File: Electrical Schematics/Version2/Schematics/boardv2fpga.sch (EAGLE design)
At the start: 132 parts, among them Q1 ASFL1

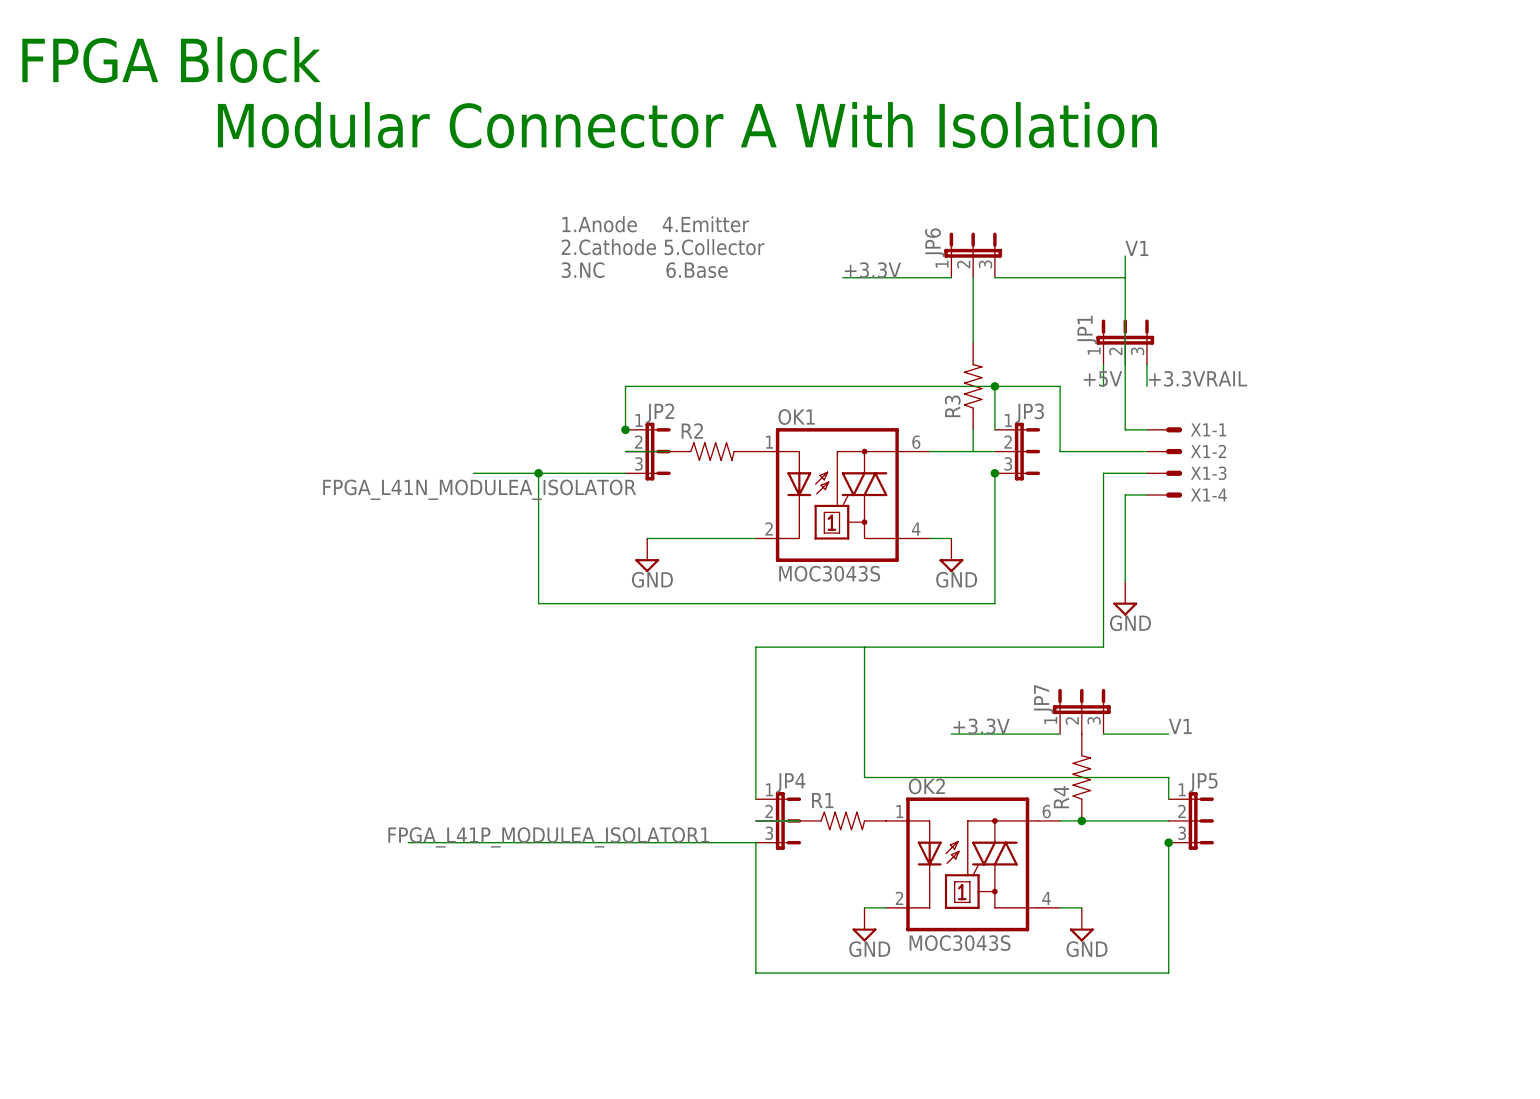
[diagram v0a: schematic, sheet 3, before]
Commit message: Fixed Grounds
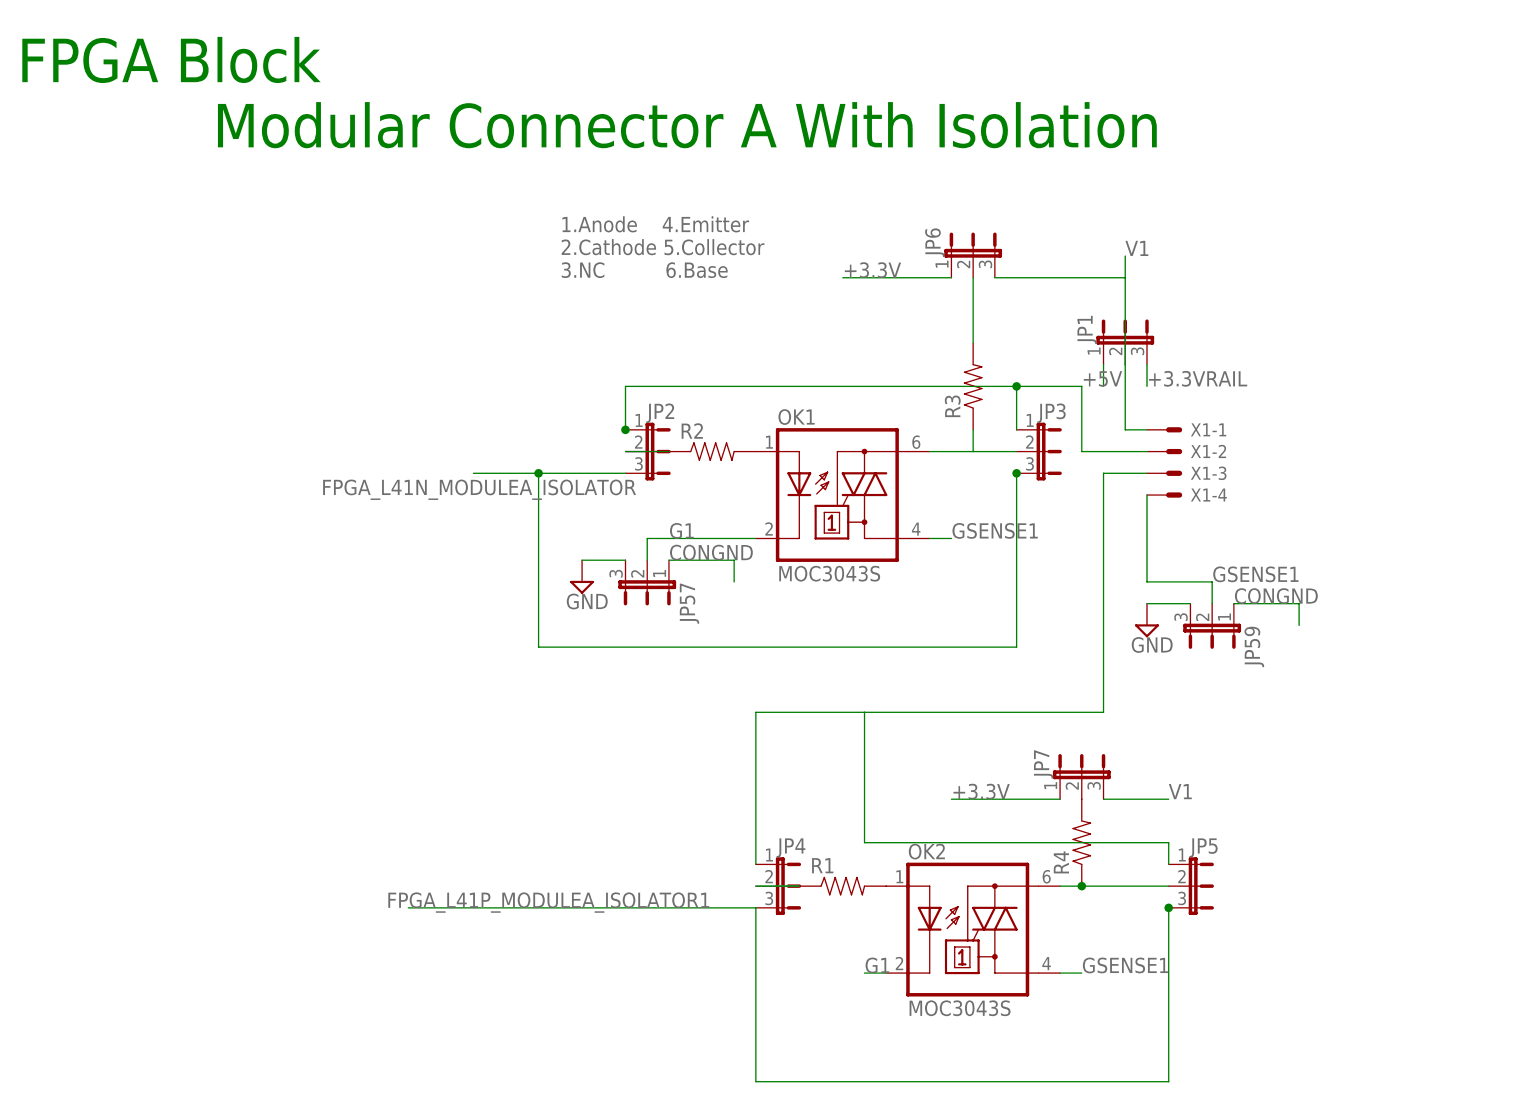
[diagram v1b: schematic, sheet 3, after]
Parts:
- added JP57, JP59, JP60, JP61, JP64, JP65, JP66, JP68, JP69, JP71, JP72, JP74, JP75, JP77, JP78, JP80: (no value), jumper:JP2E
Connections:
- new net CONGND: JP57.1, JP59.1, JP60.1, JP61.1, JP64.1, JP65.1, JP66.1, JP68.1, JP69.1, JP71.1, JP72.1, JP74.1, JP75.1, JP77.1, JP78.1, JP80.1
- new net G1: JP57.2, OK1.C, OK2.C
- new net G2: JP60.2, OK3.C, OK4.C
- new net G3: JP65.2, OK5.C, OK6.C
- new net G4: JP66.2, OK7.C, OK8.C
- new net G5: JP69.2, OK10.C, OK9.C
- new net G6: JP72.2, OK11.C, OK12.C
- new net G7: JP75.2, OK13.C, OK14.C
- new net G8: JP78.2, OK15.C, OK16.C
- new net GSENSE1: JP59.2, OK1.A1, OK2.A1, X1-4.S
- new net GSENSE2: JP61.2, OK3.A1, OK4.A1, X2-4.S
- new net GSENSE3: JP64.2, OK5.A1, OK6.A1, X3-4.S
- new net GSENSE4: JP68.2, OK7.A1, OK8.A1, X4-4.S
- new net GSENSE5: JP71.2, OK10.A1, OK9.A1, X5-4.S
- new net GSENSE6: JP74.2, OK11.A1, OK12.A1, X6-4.S
- new net GSENSE7: JP77.2, OK13.A1, OK14.A1, X7-4.S
- new net GSENSE8: JP80.2, OK15.A1, OK16.A1, X8-4.S
- net GND: now also JP57.3, JP59.3, JP60.3, JP61.3, JP64.3, JP65.3, JP66.3, JP68.3, JP69.3, JP71.3, JP72.3, JP74.3, JP75.3, JP77.3, JP78.3, JP80.3; no longer OK1.A1, OK1.C, OK10.A1, OK10.C, OK11.A1, OK11.C, OK12.A1, OK12.C, OK13.A1, OK13.C, OK14.A1, OK14.C, OK15.A1, OK15.C, OK16.A1, OK16.C, OK2.A1, OK2.C, OK3.A1, OK3.C, OK4.A1, OK4.C, OK5.A1, OK5.C, OK6.A1, OK6.C, OK7.A1, OK7.C, OK8.A1, OK8.C, OK9.A1, OK9.C, X1-4.S, X2-4.S, X3-4.S, X4-4.S, X5-4.S, X6-4.S, X7-4.S, X8-4.S
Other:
- moved on the sheet: JP11, JP12, JP14, JP18, JP19, JP21, JP25, JP26, JP28, JP3, JP32, JP33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

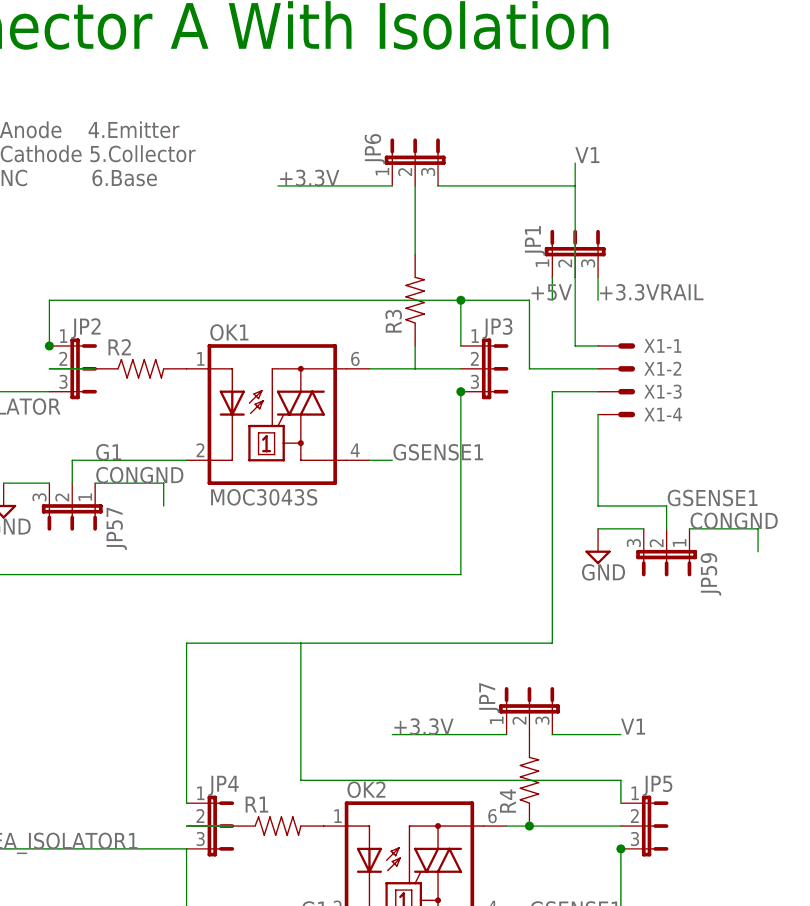
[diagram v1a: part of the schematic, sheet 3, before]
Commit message: Saved Changes
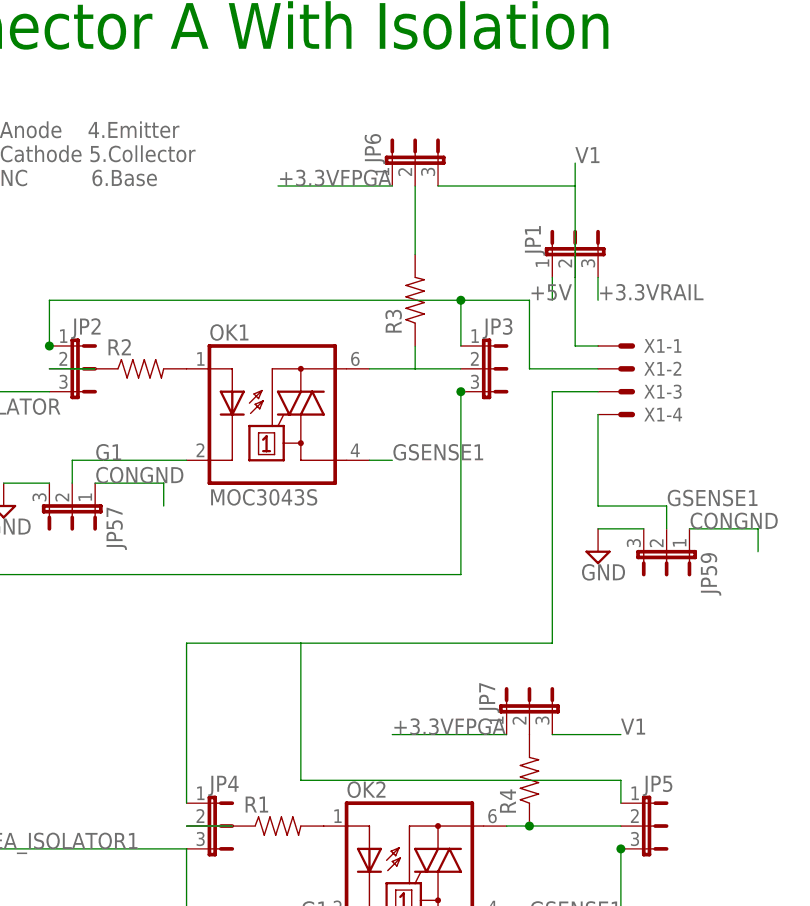
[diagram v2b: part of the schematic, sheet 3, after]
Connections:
- net +3.3V renamed +3.3VFPGA
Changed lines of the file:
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@@
 </segment>
 </net>
-<net name="+3.3V" class="0">
+<net name="+3.3VFPGA" class="0">
 <segment>
 <pinref part="JP6" gate="1" pin="1"/>
@@
 </segment>
 </net>
-<net name="+3.3V" class="0">
+<net name="+3.3VFPGA" class="0">
 <segment>
 <pinref part="JP13" gate="1" pin="1"/>
@@
 </segment>
 </net>
-<net name="+3.3V" class="0">
+<net name="+3.3VFPGA" class="0">
 <segment>
 <pinref part="JP20" gate="1" pin="1"/>
@@
 </segment>
 </net>
-<net name="+3.3V" class="0">
+<net name="+3.3VFPGA" class="0">
 <segment>
 <pinref part="JP27" gate="1" pin="1"/>
@@
 </segment>
 </net>
-<net name="+3.3V" class="0">
+<net name="+3.3VFPGA" class="0">
 <segment>
 <pinref part="JP34" gate="1" pin="1"/>
@@
 </segment>
 </net>
-<net name="+3.3V" class="0">
+<net name="+3.3VFPGA" class="0">
 <segment>
 <pinref part="JP41" gate="1" pin="1"/>
@@
 </segment>
 </net>
-<net name="+3.3V" class="0">
+<net name="+3.3VFPGA" class="0">
 <segment>
 <pinref part="JP48" gate="1" pin="1"/>
@@
 </segment>
 </net>
-<net name="+3.3V" class="0">
+<net name="+3.3VFPGA" class="0">
 <segment>
 <pinref part="JP55" gate="1" pin="1"/>
